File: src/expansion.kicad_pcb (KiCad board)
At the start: 2 copper layers, 123.1 x 100.1 mm, 123 parts, among them J1 EXPANSION, J10 Z1_Motor, J12 Z_STOP, J14 PANELDUE, J15 ESP_COMM, J16 PANEL_DUE_OUT, J17 Extruder_Heater, J18 LCD_CONN, J19 LCD_SD, J2 E1_STOP, J20 FAN2, J21 THERMISTOR2, J22 Z_PROBE, J23 FAN1, J24 THERMISTOR1, J25 FAN0, J26 ALWAYS_FAN1, J27 ALWAYS_FAN0, J28 THERMISTOR0, J29 Conn_01x02, J3 E1_Motor, J30 Conn_01x02, J31 Conn_01x02, J32 Conn_01x02, J33 Conn_01x02, J34 Conn_01x02, J36 Z1, J37 Z1, J39 X, J4 E0_STOP, J40 Y2, J41 Y1, J42 Conn_02x20_Odd_Even, J43 Bed_Connections, J5 E0_motor, J6 X_STOP, J7 X_motor, J8 Y_motor, J9 Y_STOP, M1 LOGO, M2 FID, M3 FID, M4 MOUNTING, M5 MOUNTING, M6 MOUNTING, M7 MOUNTING, Q1 DMG2305UX-13, Q2 2N7002-7-F, Q3 DMG2305UX-13, Q4 2N7002-7-F, Q5 DMG2305UX-13, Q6 2N7002-7-F, U1 SN74HCT04PWR, U2 SN74HCT04PWR, U3 SN74HCT04PWR, U4 MC74VHCT50ADTR2G, U5 74HC14

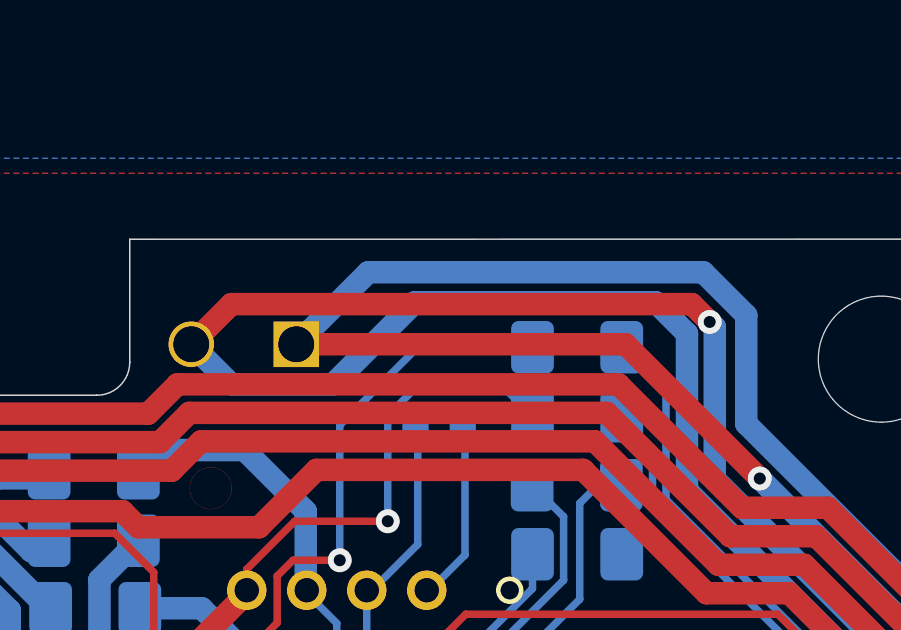
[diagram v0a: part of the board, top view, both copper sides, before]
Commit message: trace change
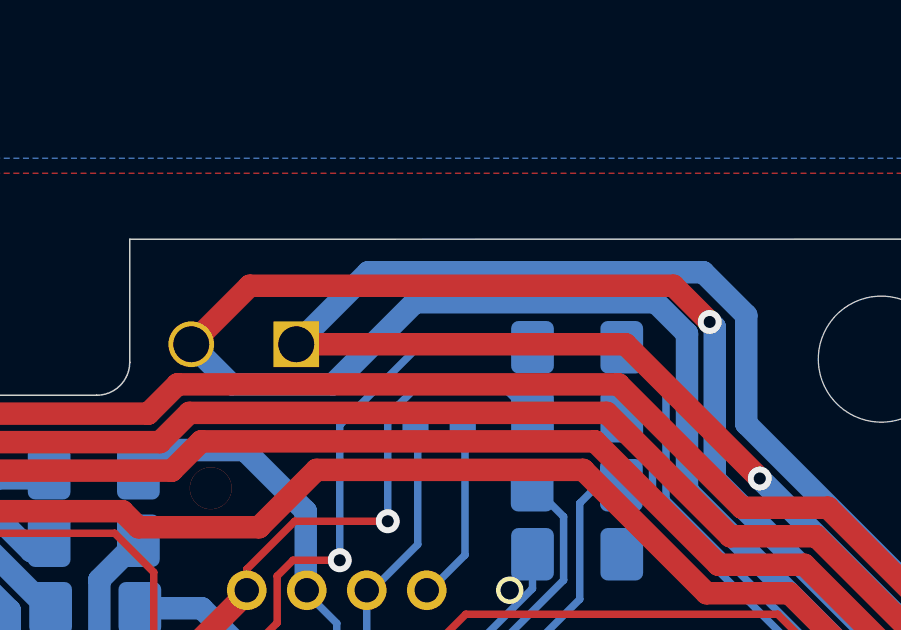
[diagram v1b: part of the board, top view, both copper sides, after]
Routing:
- net E0-: track 279.4 -> 279.9 mm
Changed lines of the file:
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@@
   (segment (start 210.864982 30.724992) (end 210.880735 30.709239) (width 0.75) (layer F.Cu) (net 6))
   (segment (start 210.880735 30.709239) (end 210.880735 30.706482) (width 0.75) (layer F.Cu) (net 6))
-  (segment (start 210.287252 30.112999) (end 210.880735 30.706482) (width 0.75) (layer F.Cu) (net 6))
-  (segment (start 193.6 31.45) (end 194.937001 30.112999) (width 0.75) (layer F.Cu) (net 6) (status 10))
-  (segment (start 194.937001 30.112999) (end 210.287252 30.112999) (width 0.75) (layer F.Cu) (net 6))
   (segment (start 157.25 88.55) (end 166.124979 79.675021) (width 0.75) (layer F.Cu) (net 6))
   (segment (start 151.75 88.55) (end 157.25 88.55) (width 0.75) (layer F.Cu) (net 6))
@@
   (segment (start 166.700011 80.599989) (end 196.955908 80.599989) (width 0.75) (layer F.Cu) (net 6))
   (via (at 199.115054 82.759135) (size 0.8) (drill 0.4) (layers F.Cu B.Cu) (net 6))
-  (via (at 210.880735 30.706482) (size 0.8) (drill 0.4) (layers F.Cu B.Cu) (net 6) (status 1000000))
+  (via (at 210.880735 30.706482) (size 0.8) (drill 0.4) (layers F.Cu B.Cu) (net 6))
+  (segment (start 209.674253 29.5) (end 210.880735 30.706482) (width 0.75) (layer F.Cu) (net 6))
+  (segment (start 193.6 31.45) (end 195.55 29.5) (width 0.75) (layer F.Cu) (net 6))
+  (segment (start 195.55 29.5) (end 209.674253 29.5) (width 0.75) (layer F.Cu) (net 6))
   (segment (start 161.214998 66.498987) (end 161.214998 70.802498) (width 0.25) (layer B.Cu) (net 8))
   (segment (start 177.552989 66.099989) (end 161.613996 66.099989) (width 0.25) (layer B.Cu) (net 8))
